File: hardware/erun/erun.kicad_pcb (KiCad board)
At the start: 2 copper layers, 10 parts, among them J1 HEIDENHAIN_MT25_TTL, J2 TRIGGER_TTL, J3 Conn_Coaxial, U1 MC3486N, U2 TXB0108DQSR, U3 MC3486N, U4 Teensy4.0, U5 LF47_TO252, U6 TXB0108DQSR, U7 MCP3301

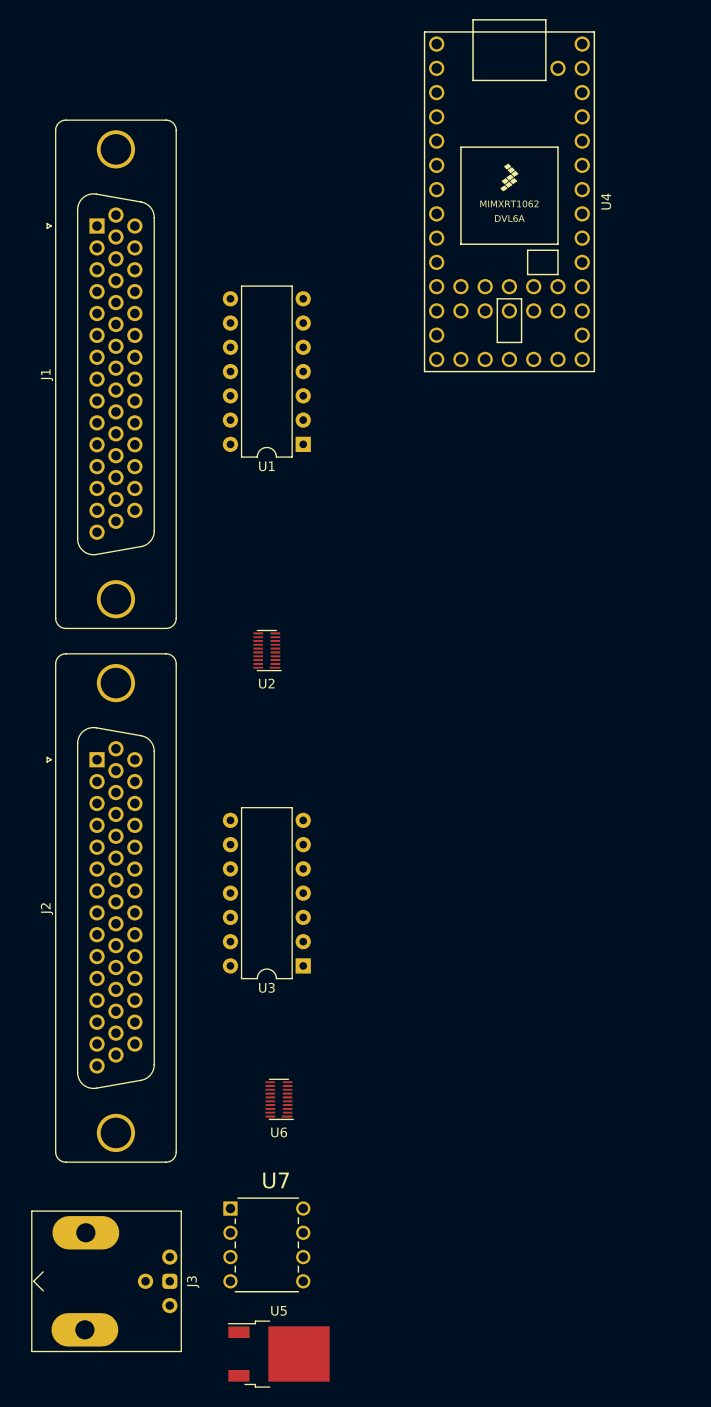
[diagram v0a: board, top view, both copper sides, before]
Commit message: Updated schematics and PCB design
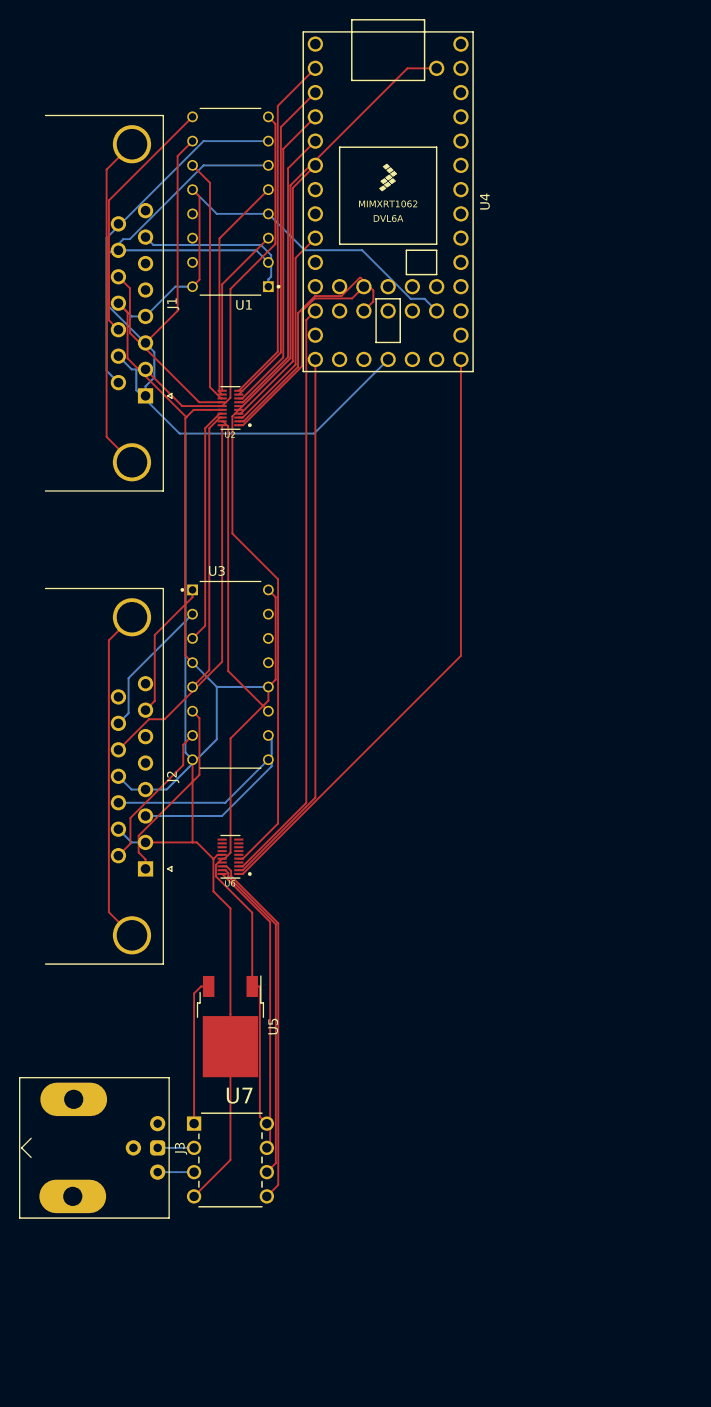
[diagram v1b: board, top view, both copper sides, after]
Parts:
- J1, J2: footprint Connector_Dsub:DSUB-44-HD_Female_Vertical_P2.29x1.98mm_MountingHoles -> Connector_Dsub:DSUB-15_Female_Horizontal_P2.77x2.84mm_EdgePinOffset7.70mm_Housed_MountingHolesOffset9.12mm
- U1, U3: footprint Package_DIP:DIP-14_W7.62mm -> MC3486N:DIP794W45P254L1969H508Q16
- U2, U6: footprint Package_SON:USON-20_2x4mm_P0.4mm -> TXB0108DQSR:SON40P400X200X55-20N
- moved U5 34.7 mm to (31.8, 114.3), turned to 270 degrees
- moved U3 31.4 mm to (31.8, 77.5), turned to 0 degrees
- moved U1 26.5 mm to (31.8, 27.9)
- moved U6 25.9 mm to (31.8, 96.5)
- moved U2 25.7 mm to (31.8, 49.5)
- moved J1 18.5 mm to (22.9, 48.3), turned to 270 degrees
- moved J3 14.0 mm to (24.1, 127.0)
- moved U4 12.7 mm to (48.3, 27.9)
- moved J2 12.5 mm to (22.9, 97.8), turned to 270 degrees
- moved U7 9.67 mm to (35.6, 132.1)
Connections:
- J3 pad 1: /ADC_INGND -> /ADC_IN5V
- J3 pad 2: /ADC_IN5V -> /ADC_INGND
- U1 pad 10: /S1_A1_HV+ -> /S1_A2_HV+
- U1 pad 11: /S1_A1_HV -> /S1_A2_HV
- U1 pad 5: /S1_A2_HV -> /S1_A1_HV
- U1 pad 6: /S1_A2_HV+ -> /S1_A1_HV+
- U1 pad 7: /S1_A2_HV- -> /S1_A1_HV-
- U1 pad 9: /S1_A1_HV- -> /S1_A2_HV-
- U3 pad 10: /S2_A1_HV+ -> /S2_A2_HV+
- U3 pad 11: /S2_A1_HV -> /S2_A2_HV
- U3 pad 5: /S2_A2_HV -> /S2_A1_HV
- U3 pad 6: /S2_A2_HV+ -> /S2_A1_HV+
- U3 pad 7: /S2_A2_HV- -> /S2_A1_HV-
- U3 pad 9: /S2_A1_HV- -> /S2_A2_HV-
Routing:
- net +5V: track 0.00 -> 185.4 mm
- net GND: track 0.00 -> 172.7 mm
- net +3V3: track 0.00 -> 97.3 mm
- net /ADC_CLK_LV: track 0.00 -> 63.8 mm
- net /ADC_CS_LV: track 0.00 -> 61.7 mm
- net /ADC_MISO_LV: track 0.00 -> 57.0 mm
- net /S2_AS_HV: track 0.00 -> 39.5 mm
- net /S1_A1_HV+: track 0.00 -> 37.8 mm
- net /ADC_CS_HV: track 0.00 -> 37.8 mm
- net /S1_A0_LV: track 0.00 -> 37.1 mm
- net /S1_A1_HV-: track 0.00 -> 36.8 mm
- net Net-(J1-Pad0): track 0.00 -> 35.5 mm
- net Net-(J2-Pad0): track 0.00 -> 35.3 mm
- net /S1_A1_LV: track 0.00 -> 34.9 mm
- net /ADC_MISO_HV: track 0.00 -> 34.5 mm
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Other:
- net class Default: clearance 0.2 -> 0.05; trace_width 0.25 -> 0.2
- rule trace_clearance: 0.2 -> 0.05

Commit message: erun updates
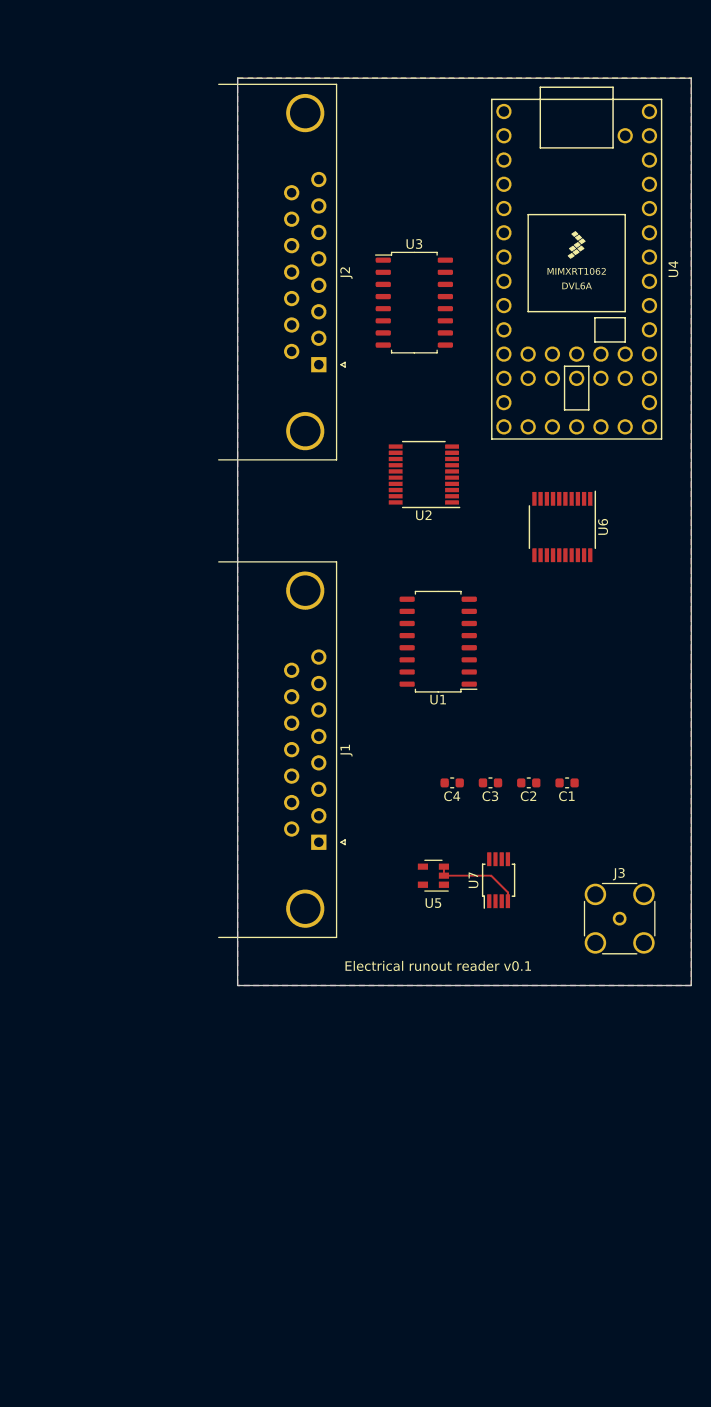
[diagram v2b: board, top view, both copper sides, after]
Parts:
- added C1: C, Capacitor_SMD:C_0603_1608Metric, F.Cu at (67.0, 88.8)
- added C2: C, Capacitor_SMD:C_0603_1608Metric, F.Cu at (63.0, 88.8)
- added C3: C, Capacitor_SMD:C_0603_1608Metric, F.Cu at (59.0, 88.8)
- added C4: C, Capacitor_SMD:C_0603_1608Metric, F.Cu at (55.0, 88.8)
- J3: footprint Connector_Coaxial:BNC_Amphenol_031-6575_Horizontal -> Connector_Coaxial:SMA_Amphenol_132134-14_Vertical
- U1, U3: footprint MC3486N:DIP794W45P254L1969H508Q16 -> Package_SO:SOIC-16_4.55x10.3mm_P1.27mm
- U2, U6: footprint TXB0108DQSR:SON40P400X200X55-20N -> Package_SO:TSSOP-20_4.4x6.5mm_P0.65mm
- U5: value LF47_TO252 -> TPS793475-EP; footprint Package_TO_SOT_SMD:TO-252-2 -> Package_TO_SOT_SMD:SOT-23-5
- U7: footprint MCP3301:DIP254P762X432-8 -> Package_SO:MSOP-8_3x3mm_P0.65mm
- moved J2 55.8 mm to (41.0, 45.0)
- moved J3 54.0 mm to (72.5, 103.0), turned to 0 degrees
- moved U1 50.9 mm to (53.5, 74.0)
- moved J1 50.1 mm to (41.0, 95.0)
- moved U6 49.0 mm to (66.5, 62.0), turned to 270 degrees
- moved U3 43.5 mm to (51.0, 38.5)
- moved U7 41.0 mm to (59.8, 99.0), turned to 90 degrees
- moved U5 26.5 mm to (53.0, 98.5), turned to 180 degrees
- moved U2 21.4 mm to (52.0, 56.5)
- moved U4 21.0 mm to (68.0, 35.0)
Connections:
- J1 pad 0: Net-(J1-Pad0) -> GND
- J2 pad 0: Net-(J2-Pad0) -> GND
- U2 pad 6: Net-(U2-Pad6) -> +3V3
- U4 pad 1: Net-(U4-Pad1) -> GND
- U4 pad 31: Net-(U4-Pad31) -> +3V3
- U4 pad 32: Net-(U4-Pad32) -> GND
- U4 pad 34: +3V3 -> +5V
- U4 pad 35: +5V -> Net-(U4-Pad35)
- U5 pad 3: /ADC_REF -> GND
- U6 pad 6: /LLC_OE -> +3V3
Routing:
- net +5V: track 185.4 -> 0.00 mm
- net GND: track 172.7 -> 9.30 mm
- net +3V3: track 97.3 -> 0.00 mm
- net /ADC_CLK_LV: track 63.8 -> 0.00 mm
- net /ADC_CS_LV: track 61.7 -> 0.00 mm
- net /ADC_MISO_LV: track 57.0 -> 0.00 mm
- net /S2_AS_HV: track 39.5 -> 0.00 mm
- net /S1_A1_HV+: track 37.8 -> 0.00 mm
- net /ADC_CS_HV: track 37.8 -> 0.00 mm
- net /S1_A0_LV: track 37.1 -> 0.00 mm
- net /S1_A1_HV-: track 36.8 -> 0.00 mm
- net Net-(J1-Pad0): track 35.5 -> 0.00 mm
- net Net-(J2-Pad0): track 35.3 -> 0.00 mm
- net /S1_A1_LV: track 34.9 -> 0.00 mm
- net /ADC_MISO_HV: track 34.5 -> 0.00 mm
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- added copper zone on B.Cu, net GND
- added copper zone on F.Cu, net GND
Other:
- board outline added: 47.5 x 95 mm
- board text added: "Electrical runout reader v0.1"
